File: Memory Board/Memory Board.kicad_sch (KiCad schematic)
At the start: 40 parts, among them IC1 W25Q01JVZEIQ, IC2 MCP2557FDT-H_MNY, J1 USB4056-03-A_REVA2, J2 Conn_01x04_Socket, J3 Conn_01x04_Socket, J4 Conn_01x04_Socket, SW1 SW_SPST, U1 STM32G473CBTx, U2 LD1117S33TR_SOT223, U3 LD1117S50TR_SOT223, X1 ECS-2520MV-xxx-xx

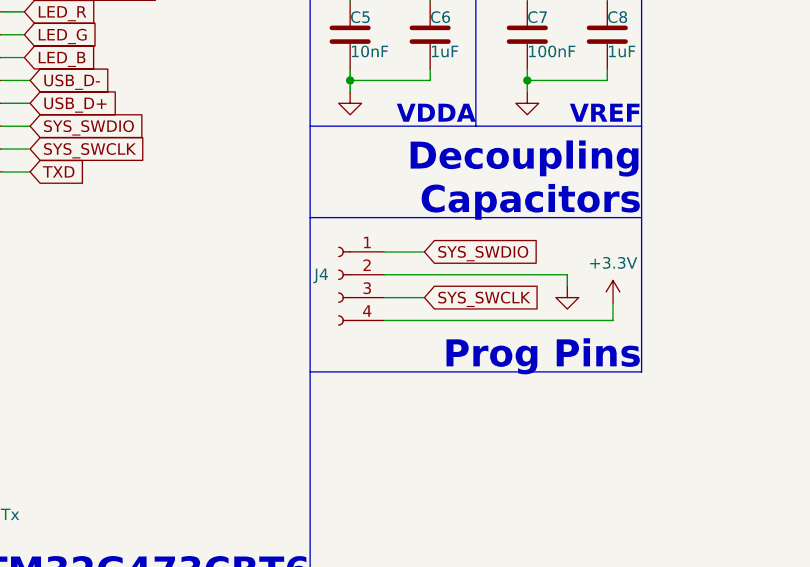
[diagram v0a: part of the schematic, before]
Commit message: Layout work
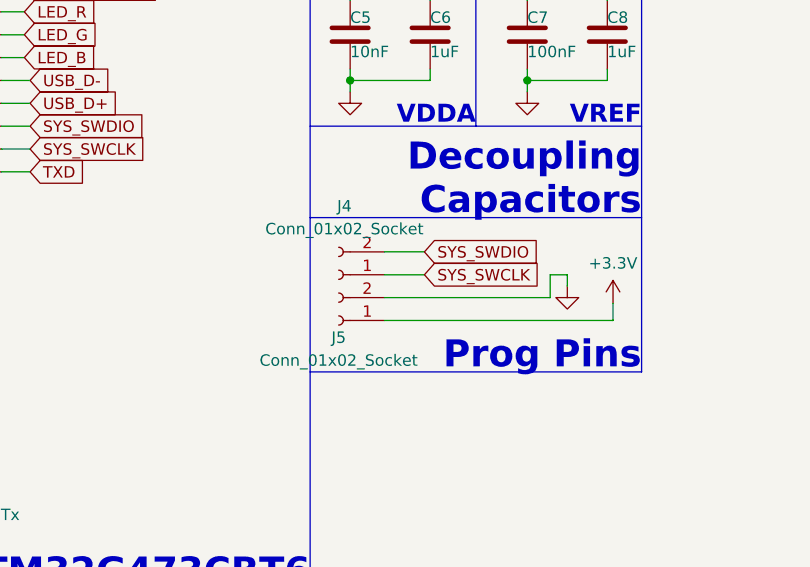
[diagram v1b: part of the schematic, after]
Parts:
- removed J4: Conn_01x04_Socket, Connector_PinHeader_2.54mm:PinHeader_1x04_P2.54mm_Vertical, symbol Connector:Conn_01x04_Socket
- added J4, J5: Conn_01x02_Socket, Connector_PinHeader_2.54mm:PinHeader_1x02_P2.54mm_Vertical, symbol Connector:Conn_01x02_Socket
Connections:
- net +3.3V: now also J5.1 (Pin_1)
- net GND: now also J5.2 (Pin_2)
- net SYS_SWCLK: now also J4.1 (Pin_1)
- net SYS_SWDIO: now also J4.2 (Pin_2)
